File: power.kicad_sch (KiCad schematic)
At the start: 14 parts, among them J1 USB_C_Receptacle_USB2.0_16P, U40 RP2040, U41 W25Q128JVS, U42 MIC5219-3.3YM5, Y1 12MHz

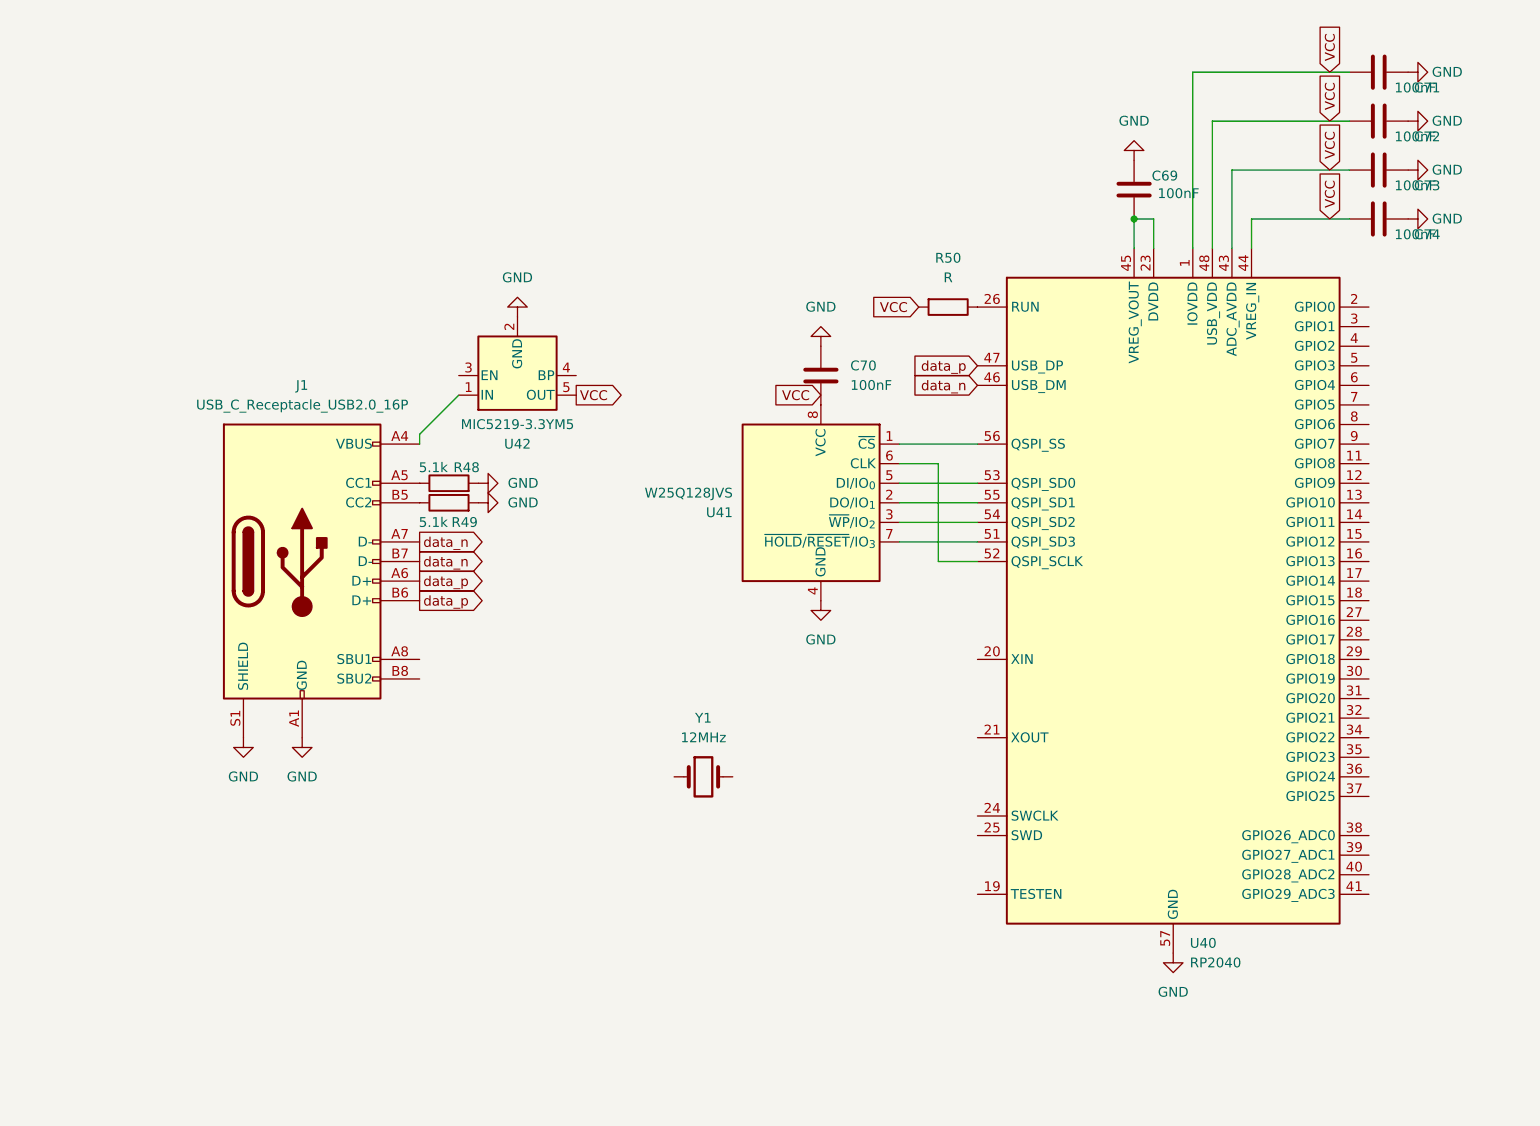
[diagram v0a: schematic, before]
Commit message: Updated: power
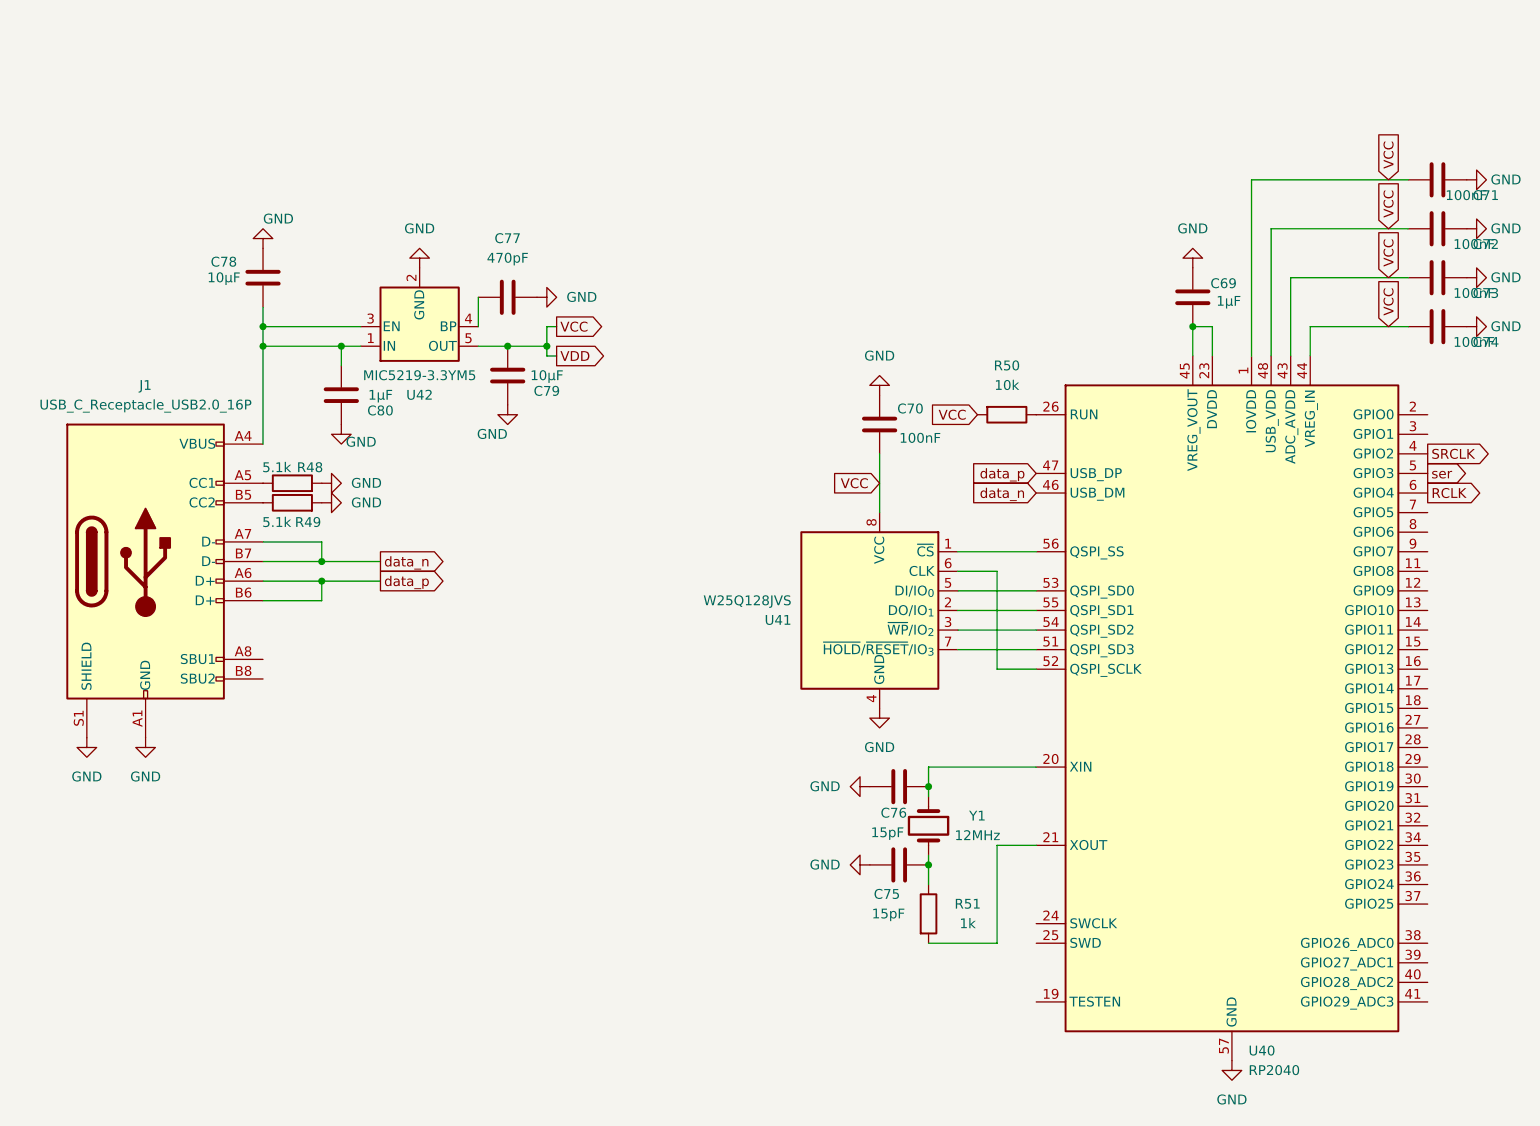
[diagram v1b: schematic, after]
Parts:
- added C75, C76: 15pF, symbol Device:C
- added C77: 470pF, symbol Device:C
- added C78, C79: 10µF, symbol Device:C
- added C80: 1µF, symbol Device:C
- added R51: 1k, Resistor_SMD:R_1206_3216Metric_Pad1.30x1.75mm_HandSolder, symbol Device:R
- C69: value 100nF -> 1µF
- R48, R49: footprint (none) -> Resistor_SMD:R_1206_3216Metric_Pad1.30x1.75mm_HandSolder
- R50: value R -> 10k; footprint (none) -> Resistor_SMD:R_1206_3216Metric_Pad1.30x1.75mm_HandSolder
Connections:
- net GND: now also C75.2, C76.2, C77.2, C78.2, C79.2, C80.2
- net VCC: now also C70.2, U41.8 (VCC), C79.1
- net at J1.A4 (VBUS), J1.A9 (VBUS), J1.B4 (VBUS)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: now also U42.3 (EN), C78.1, C80.1
- net at U40.20 (XIN): now also Y1.1, C76.1
- net at U40.21 (XOUT): now also R51.2
- net SRCLK: now reaches U40.4 (GPIO2)
- net ser: now reaches U40.5 (GPIO3)
- net RCLK: now reaches U40.6 (GPIO4)
- net at U42.4 (BP): now also C77.1
- net at Y1.2: now also C75.1, R51.1
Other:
- moved on the sheet: C69, C70, C71, C72, C73, C74, J1, R48, R49, R50, U40, U41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
